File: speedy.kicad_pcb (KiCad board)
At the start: 2 copper layers, 49.4 x 49.4 mm, 131 parts, among them Q1 2N7002, Q2 2N7002, SW1 DFU, SW2 PushButton, U1 STM32F415RGT6, U10 INA213-SC70, U11 LT1965, U12 MCP73831, U13 DRV8839, U14 DRV8839, U2 NUF2042VX6, U3 MPU-9250, U4 MS5611-01BA, U5 VL6180X, U6 NRF24L01+, U7 LT1965, U8 LT1965, U9 LTC2955DDB-1, X1 16Mhz 10ppm

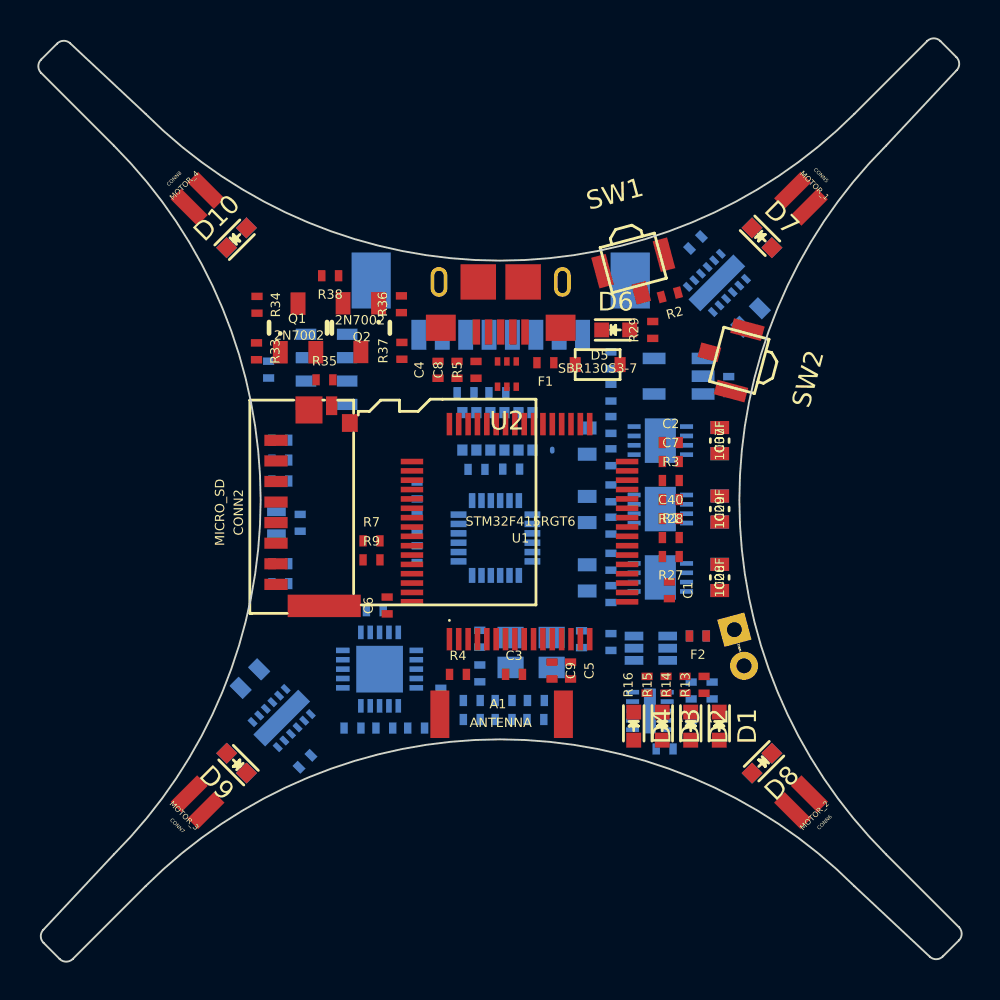
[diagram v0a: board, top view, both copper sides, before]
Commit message: Update form to square PCB, place components and update 3D models
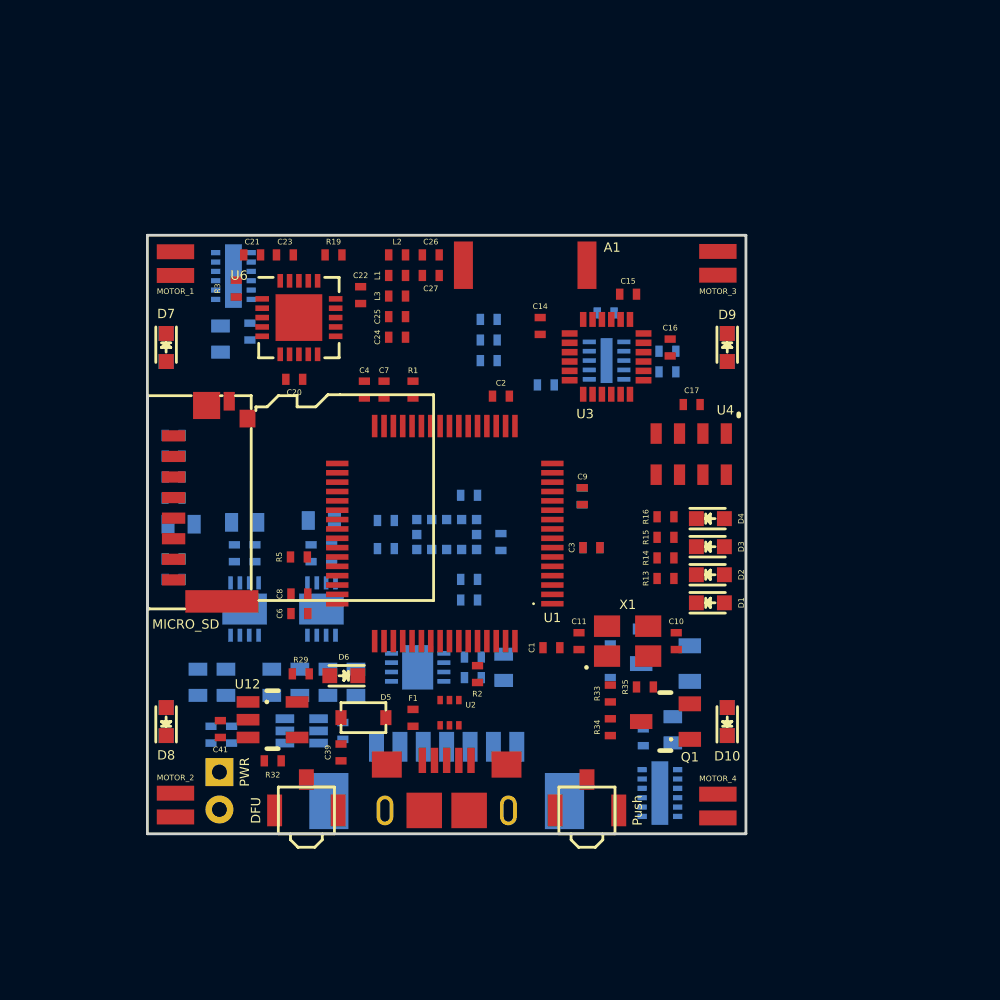
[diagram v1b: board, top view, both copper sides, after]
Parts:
- C10, C11, C14, C15, C16, C17, C20, C21, C22, C23, C24, C25, C26, C27, C39, C41, L1, L2, L3, R19, R32, U12, U3, U4, U6, X1: moved to F.Cu
- C18: value 0.1uF -> 4.7uF
- C19: value 4.7uF -> 0.1uF
- C28, C29, C37, C40, C5, F2, Q2, R27, R28, R36, R37, R38, R4, R7, R9: moved to B.Cu
- CONN1: value JTAG -> SWD/DEBUG; footprint _connectors:_Molex-PicoBlade-SMD-8 -> _connectors:_Molex-PicoBlade-SMD-7
- R17, R18: value 47k -> 10k
- SW2: value PushButton -> Push
- U5: value VL6180X -> VL53L0X; footprint _sensors:VL6180X -> _sensors:ST-VL53L0X
- moved CONN8 42.8 mm to (160.2, 121.4), turned to 270 degrees
- moved CONN7 40.0 mm to (160.2, 92.3), turned to 90 degrees
- moved D10 36.8 mm to (160.7, 116.8), turned to 90 degrees
- moved D14 36.8 mm to (160.7, 116.8), turned to 90 degrees
- moved D9 34.4 mm to (160.7, 96.8), turned to 270 degrees
- moved D13 34.4 mm to (160.7, 96.9), turned to 270 degrees
- moved SW1 34.1 mm to (138.2, 121.6), turned to 180 degrees
- moved CONN5 33.6 mm to (131.2, 92.4), turned to 90 degrees
- moved CONN6 33.4 mm to (131.2, 121.3), turned to 270 degrees
- moved C41 32.8 mm to (133.6, 117.2)
- moved D11 32.4 mm to (130.7, 96.8), turned to 270 degrees
- moved D7 32.4 mm to (130.7, 96.8), turned to 270 degrees
- moved D8 31.9 mm to (130.7, 116.8), turned to 90 degrees
- moved D12 31.9 mm to (130.7, 116.9), turned to 90 degrees
- moved C37 30.7 mm to (132.3, 114.8), turned to 270 degrees
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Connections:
- CONN1 pad 4: /STM32F4_TRST -> /STM32F4_SWDIO
- CONN1 pad 5: /STM32F4_TDI -> /STM32F4_SWCLK
- CONN1 pad 6: /STM32F4_TDO -> /UART3_TX
- CONN1 pad 7: /STM32F4_TMS -> /UART3_RX
- R17 pad 2: Net-(R17-Pad2) -> /TOF_XSHUT
- R18 pad 2: Net-(R18-Pad2) -> /TOF_GPIO1
- U1 pad 14: Net-(U1-Pad14) -> /TOF_XSHUT
- U1 pad 29: /NRF24L01+_INT -> /UART3_TX
- U1 pad 30: /NRF24L01+_EN -> /UART3_RX
- U1 pad 46: /STM32F4_TMS -> /STM32F4_SWDIO
- U1 pad 49: /STM32F4_TCK -> /STM32F4_SWCLK
- U1 pad 50: /STM32F4_TDI -> /TOF_GPIO1
- U1 pad 55: /STM32F4_TDO -> /NRF24L01+_INT
- U1 pad 56: /STM32F4_TRST -> /NRF24L01+_EN
- U5 pad 1: Net-(R18-Pad2) -> VCCA
- U5 pad 10: VCCA -> /I2C1_SCL
- U5 pad 11: Net-(U5-Pad11) -> VCCA
- U5 pad 2: Net-(U5-Pad2) -> GND
- U5 pad 3: Net-(U5-Pad3) -> GND
- U5 pad 4: Net-(R17-Pad2) -> GND
- U5 pad 5: /I2C1_SCL -> /TOF_XSHUT
- U5 pad 6: /I2C1_SDA -> GND
- U5 pad 7: Net-(U5-Pad7) -> /TOF_GPIO1
- U5 pad 8: VCCA -> Net-(U5-Pad8)
- U5 pad 9: GND -> /I2C1_SDA
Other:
- board size 49.4 x 49.4 mm -> 32 x 32 mm
